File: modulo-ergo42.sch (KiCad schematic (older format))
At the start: 38 parts, among them J1 AudioJack4_Ground, J2 AudioJack4_Ground, J3 AudioJack4_Ground, J4 AudioJack4_Ground, SW1 SW_Push, SW10 SW_Push, SW11 SW_Push, SW12 SW_Push, SW13 SW_Push, SW14 SW_Push, SW15 SW_Push, SW16 SW_Push, SW17 SW_Push, SW18 SW_Push, SW19 SW_Push, SW2 SW_Push, SW20 SW_Push, SW21 SW_Push, SW22 SW_Push, SW23 SW_Push, SW24 SW_Push, SW25 SW_Push, SW26 SW_Push, SW27 SW_Push, SW28 SW_Push, SW29 SW_DIP_x02, SW3 SW_Push, SW4 SW_Push, SW5 SW_Push, SW6 SW_Push, SW7 SW_Push, SW8 SW_Push, SW9 SW_Push, U1 TCA9555PWR, U2 TCA9555PWR

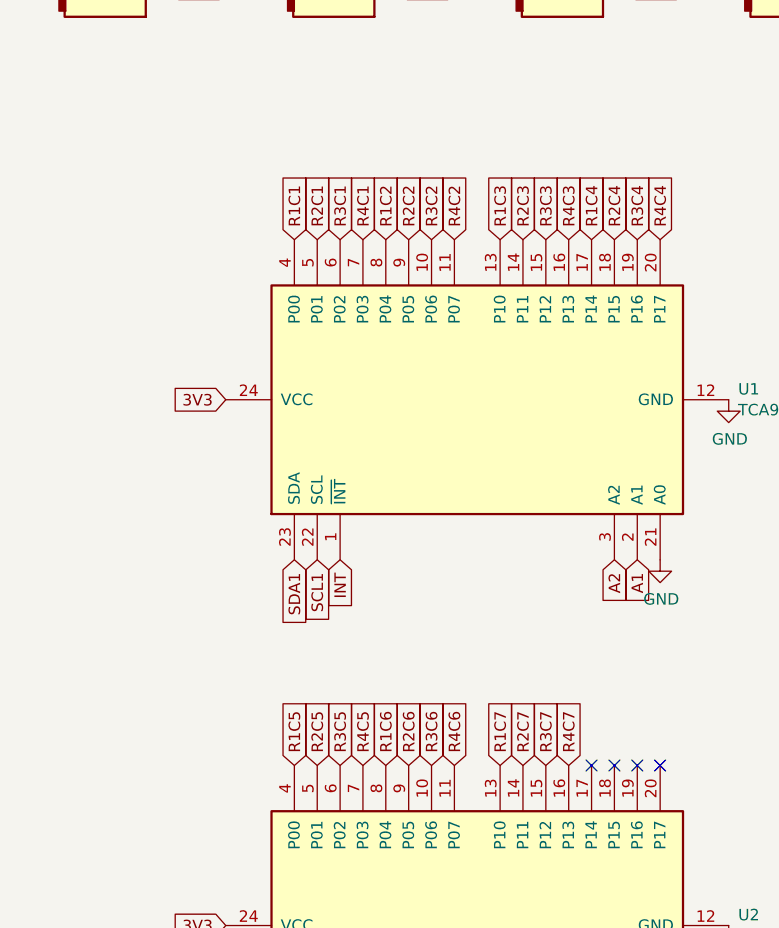
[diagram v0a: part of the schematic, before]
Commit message: Re-place parts for drill
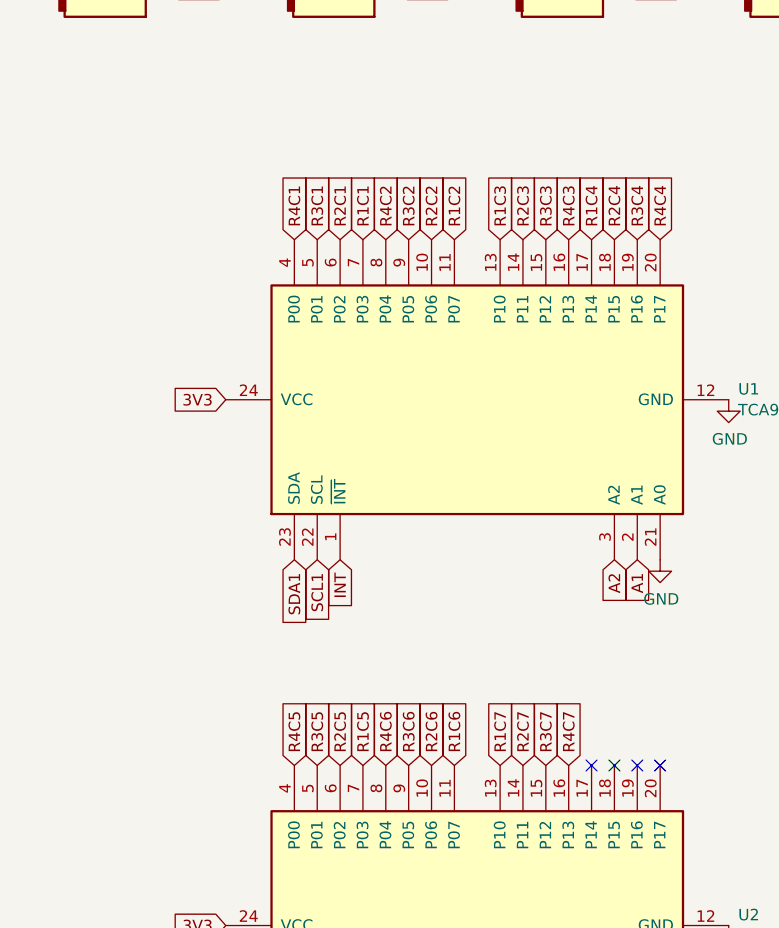
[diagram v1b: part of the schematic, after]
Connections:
- net R1C1: now also U1.7 (P03); no longer U1.4 (P00)
- net R1C2: now also U1.11 (P07); no longer U1.8 (P04)
- net R1C5: now also U2.7 (P03); no longer U2.4 (P00)
- net R1C6: now also U2.11 (P07); no longer U2.8 (P04)
- net R2C1: now also U1.6 (P02); no longer U1.5 (P01)
- net R2C2: now also U1.10 (P06); no longer U1.9 (P05)
- net R2C5: now also U2.6 (P02); no longer U2.5 (P01)
- net R2C6: now also U2.10 (P06); no longer U2.9 (P05)
- net R3C1: now also U1.5 (P01); no longer U1.6 (P02)
- net R3C2: now also U1.9 (P05); no longer U1.10 (P06)
- net R3C5: now also U2.5 (P01); no longer U2.6 (P02)
- net R3C6: now also U2.9 (P05); no longer U2.10 (P06)
- net R4C1: now also U1.4 (P00); no longer U1.7 (P03)
- net R4C2: now also U1.8 (P04); no longer U1.11 (P07)
- net R4C5: now also U2.4 (P00); no longer U2.7 (P03)
- net R4C6: now also U2.8 (P04); no longer U2.11 (P07)
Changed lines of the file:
@@
 EESchema Schematic File Version 4
+LIBS:modulo-ergo42-cache
 EELAYER 26 0
 EELAYER END
@@
 NoConn ~ 3350 5800
 NoConn ~ 3150 5800
+Text GLabel 2050 3500 1    50   Input ~ 0
+R1C1
+Text GLabel 2450 3500 1    50   Input ~ 0
+R1C2
+Text GLabel 1950 3500 1    50   Input ~ 0
+R2C1
+Text GLabel 1850 3500 1    50   Input ~ 0
+R3C1
 Text GLabel 1750 3500 1    50   Input ~ 0
-R1C1
+R4C1
+Text GLabel 2350 3500 1    50   Input ~ 0
+R2C2
+Text GLabel 2250 3500 1    50   Input ~ 0
+R3C2
 Text GLabel 2150 3500 1    50   Input ~ 0
-R1C2
-Text GLabel 1850 3500 1    50   Input ~ 0
-R2C1
-Text GLabel 1950 3500 1    50   Input ~ 0
-R3C1
-Text GLabel 2050 3500 1    50   Input ~ 0
-R4C1
-Text GLabel 2250 3500 1    50   Input ~ 0
-R2C2
-Text GLabel 2350 3500 1    50   Input ~ 0
-R3C2
-Text GLabel 2450 3500 1    50   Input ~ 0
 R4C2
 Text GLabel 2650 3500 1    50   Input ~ 0
@@
 Text GLabel 3350 3500 1    50   Input ~ 0
 R4C4
+Text GLabel 2050 5800 1    50   Input ~ 0
+R1C5
+Text GLabel 1950 5800 1    50   Input ~ 0
+R2C5
+Text GLabel 1850 5800 1    50   Input ~ 0
+R3C5
 Text GLabel 1750 5800 1    50   Input ~ 0
-R1C5
-Text GLabel 1850 5800 1    50   Input ~ 0
-R2C5
-Text GLabel 1950 5800 1    50   Input ~ 0
-R3C5
-Text GLabel 2050 5800 1    50   Input ~ 0
 R4C5
+Text GLabel 2450 5800 1    50   Input ~ 0
+R1C6
+Text GLabel 2350 5800 1    50   Input ~ 0
+R2C6
+Text GLabel 2250 5800 1    50   Input ~ 0
+R3C6
 Text GLabel 2150 5800 1    50   Input ~ 0
-R1C6
-Text GLabel 2250 5800 1    50   Input ~ 0
-R2C6
-Text GLabel 2350 5800 1    50   Input ~ 0
-R3C6
-Text GLabel 2450 5800 1    50   Input ~ 0
 R4C6
 Text GLabel 2650 5800 1    50   Input ~ 0

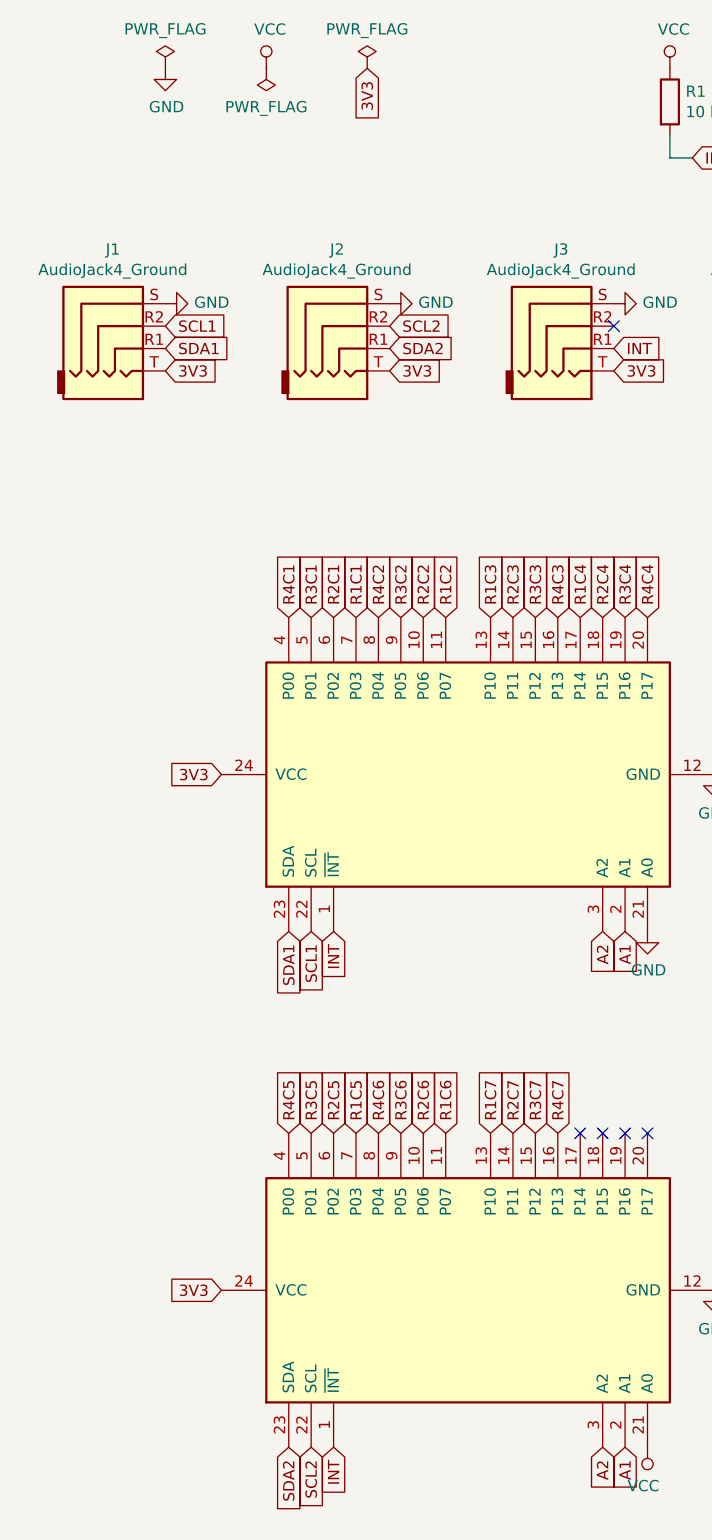
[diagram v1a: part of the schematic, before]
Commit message: Fix schematics
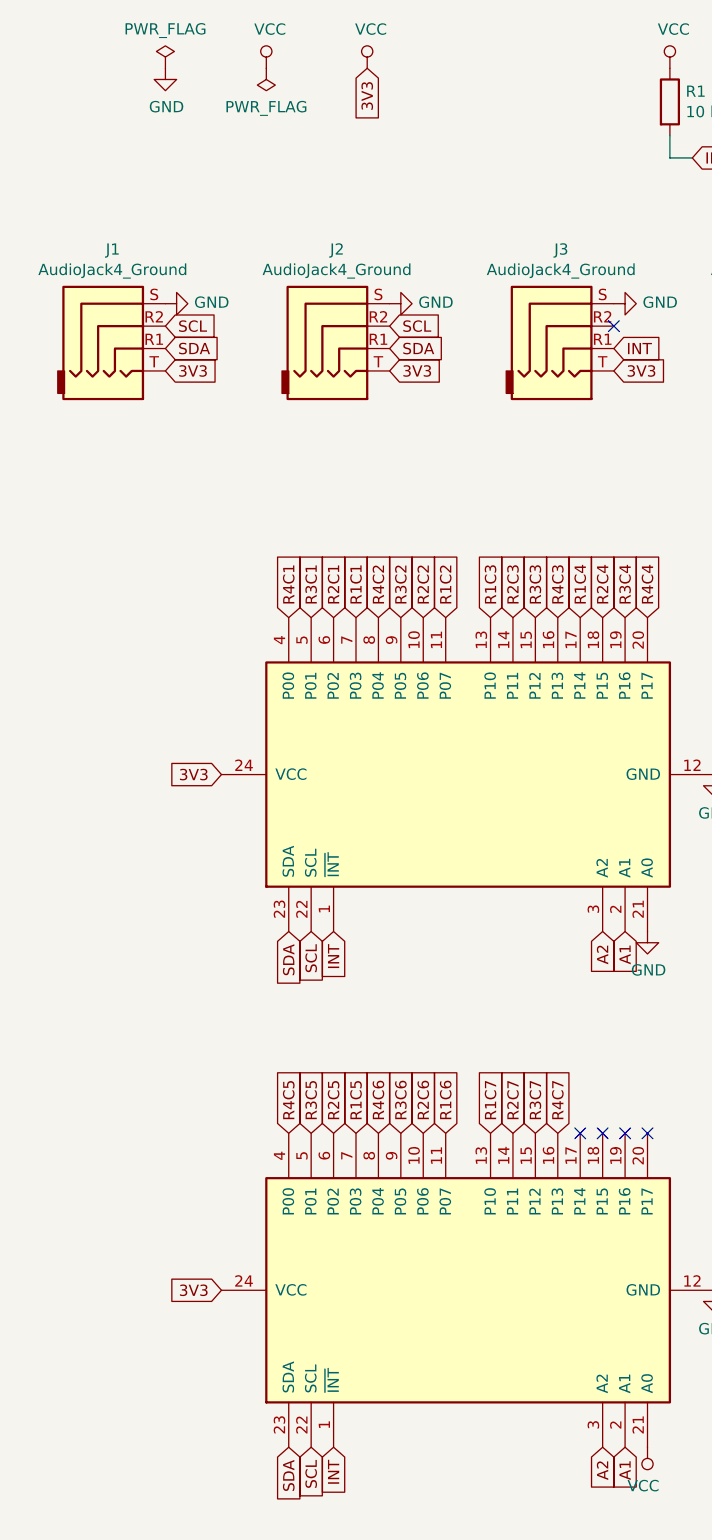
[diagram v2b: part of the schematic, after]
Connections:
- net 3V3 is gone; now on net VCC: J1.T, J2.T, J3.T, J4.T, U1.24 (VCC), U2.24 (VCC)
- net SCL2 is gone; now on net SCL: J2.R2, U2.22 (SCL)
- net SDA2 is gone; now on net SDA: J2.R1, U2.23 (SDA)
- net SCL1 renamed SCL
- net SDA1 renamed SDA
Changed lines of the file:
@@
 $EndComp
 Text GLabel 1200 2200 2    50   Input ~ 0
-SCL1
+SCL
 Text GLabel 1200 2300 2    50   Input ~ 0
-SDA1
+SDA
 Text GLabel 2200 2200 2    50   Input ~ 0
-SCL2
+SCL
 Text GLabel 2200 2300 2    50   Input ~ 0
-SDA2
+SDA
 $Comp
 L power:GND #PWR08
@@
 	3450 1450 3550 1450
 Text GLabel 1850 4900 3    50   Input ~ 0
-SCL1
+SCL
 Text GLabel 1750 4900 3    50   Input ~ 0
-SDA1
+SDA
 Text GLabel 1850 7200 3    50   Input ~ 0
-SCL2
+SCL
 Text GLabel 1750 7200 3    50   Input ~ 0
-SDA2
+SDA
 $Comp
 L power:GND #PWR06
@@
 Text GLabel 9350 5400 3    50   Input ~ 0
 R4C7
-$Comp
-L power:PWR_FLAG #FLG03
-U 1 1 5BC41E23
-P 2100 1050
-F 0 "#FLG03" H 2100 1125 50  0001 C CNN
-F 1 "PWR_FLAG" H 2100 1224 50  0000 C CNN
-F 2 "" H 2100 1050 50  0001 C CNN
-F 3 "~" H 2100 1050 50  0001 C CNN
-	1    2100 1050
-	1    0    0    -1
-$EndComp
 Text GLabel 2100 1050 3    50   Input ~ 0
 3V3
@@
 Text GLabel 4200 2400 2    50   Input ~ 0
 3V3
+$Comp
+L power:VCC #PWR0101
+U 1 1 5BCCB118
+P 2100 1050
+F 0 "#PWR0101" H 2100 900 50  0001 C CNN
+F 1 "VCC" H 2117 1223 50  0000 C CNN
+F 2 "" H 2100 1050 50  0001 C CNN
+F 3 "" H 2100 1050 50  0001 C CNN
+	1    2100 1050
+	1    0    0    -1
+$EndComp
 $EndSCHEMATC
